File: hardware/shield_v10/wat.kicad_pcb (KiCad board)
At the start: 2 copper layers, 41 parts, among them P101 INTEN_1_V, P102 CAUDAL_1, P103 V_IN, P104 INTEN_1_I, P105 PRESION_1, P106 18b20, P107 INTEN_2_V, P108 INTEN_2_I, P109 LCD_I2C, P110 ARD_DI_06, P111 ARD_ALI_04, P112 ARD_AN_I2C, U101 ESP-12, U102 Recom-rd, U103 RO-1224S, U104 LM1117, U105 mp-1584

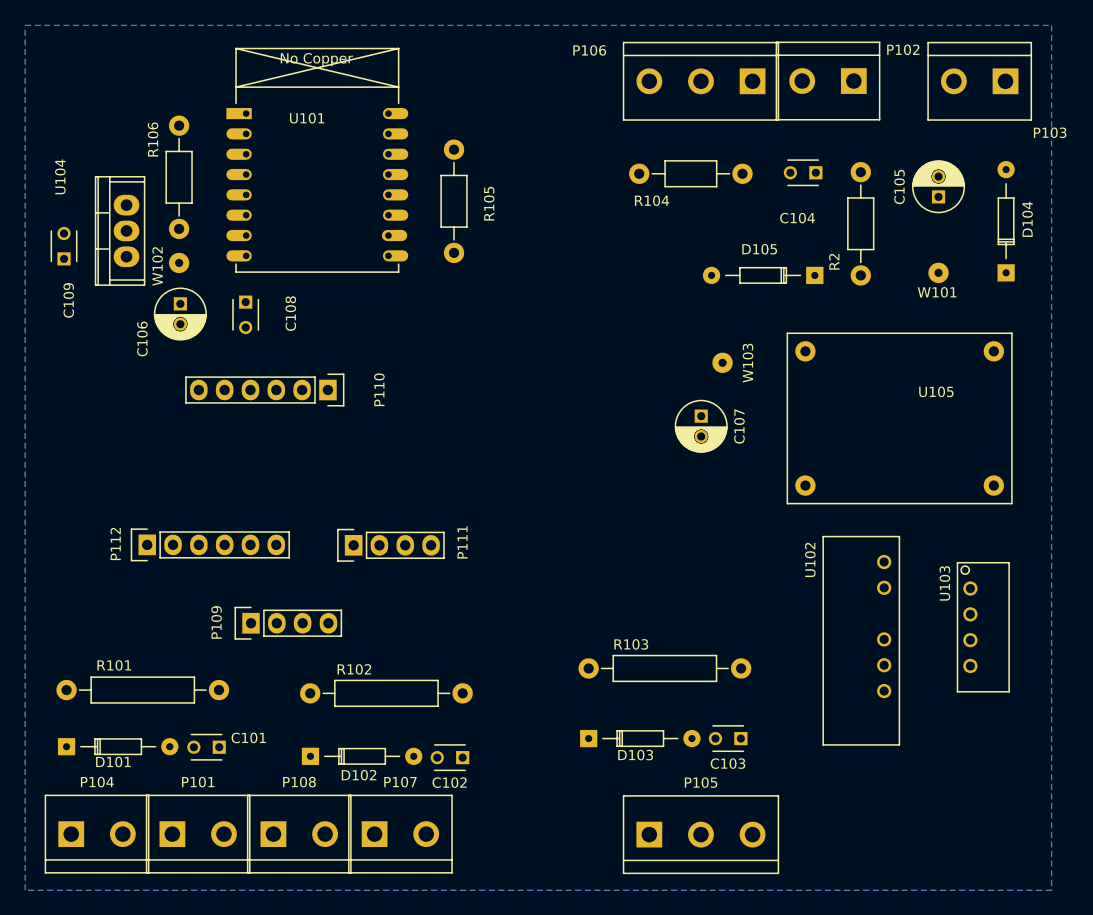
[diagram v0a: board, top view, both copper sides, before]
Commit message: [pcb] beta de la pcb
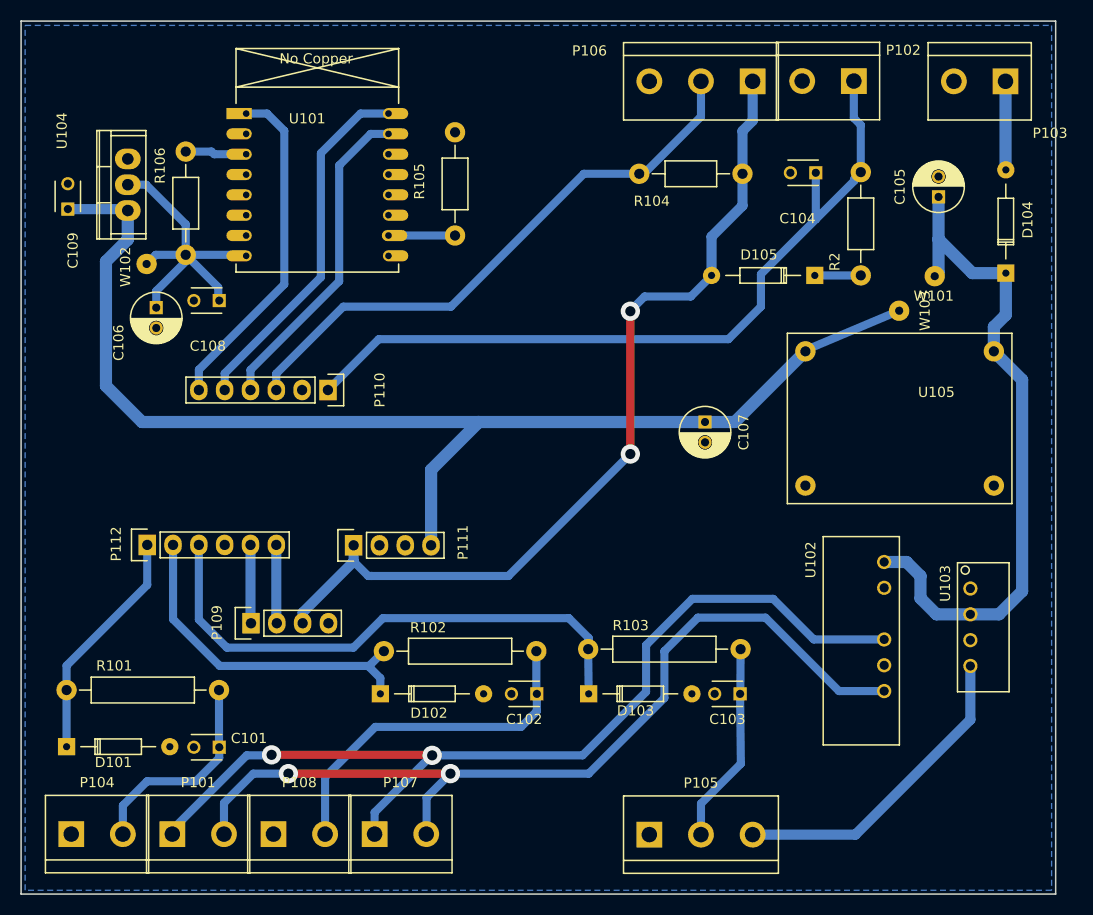
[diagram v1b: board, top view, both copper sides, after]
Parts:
- moved W103 18.1 mm to (175.0, 72.1)
- moved C102 9.63 mm to (139.3, 109.8)
- moved D102 9.22 mm to (124.0, 109.8)
- moved R105 8.45 mm to (131.3, 64.7), turned to 90 degrees
- moved R102 8.35 mm to (124.3, 105.6)
- moved C109 4.91 mm to (93.2, 62.1)
- moved U104 4.55 mm to (99.1, 59.7)
- moved C103 4.40 mm to (159.3, 109.8)
- moved D103 4.40 mm to (144.4, 109.8)
- moved W102 3.20 mm to (101.0, 67.5)
- moved R106 2.63 mm to (104.8, 66.6)
- moved C108 2.60 mm to (108.1, 71.1), turned to 180 degrees
- moved C106 2.40 mm to (101.9, 71.8)
- moved R103 1.90 mm to (144.4, 105.4)
- moved C107 0.69 mm to (155.9, 83.0)
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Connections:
- P110 pad 4: /e_tx -> /e_rx
- P110 pad 5: /e_rx -> /e_tx
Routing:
- net /Var_8V: track 0.00 -> 121.7 mm
- net /-15_voltios: track 0.00 -> 94.4 mm, vias 0 -> 2
- net /+15_voltios: track 0.00 -> 88.2 mm, vias 0 -> 2
- net /Vpc_5V: track 0.00 -> 87.0 mm, vias 0 -> 2
- net /caudal_1: track 0.00 -> 77.2 mm
- net /Vin_12V: track 0.00 -> 66.8 mm
- net /18b20: track 0.00 -> 57.4 mm
- net /presion_1: track 0.00 -> 54.4 mm
- net /e_tx: track 0.00 -> 35.5 mm
- net Net-(C102-Pad1): track 0.00 -> 35.1 mm
- net /intensidad_2: track 0.00 -> 33.8 mm
- net /e_rst: track 0.00 -> 33.4 mm
- net /Ves_3V3: track 0.00 -> 32.8 mm
- net /e_rx: track 0.00 -> 31.9 mm
- net /+24_voltios: track 0.00 -> 31.4 mm
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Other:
- board outline added: 101.8 x 85.9 mm
